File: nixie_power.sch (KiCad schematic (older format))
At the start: 17 parts

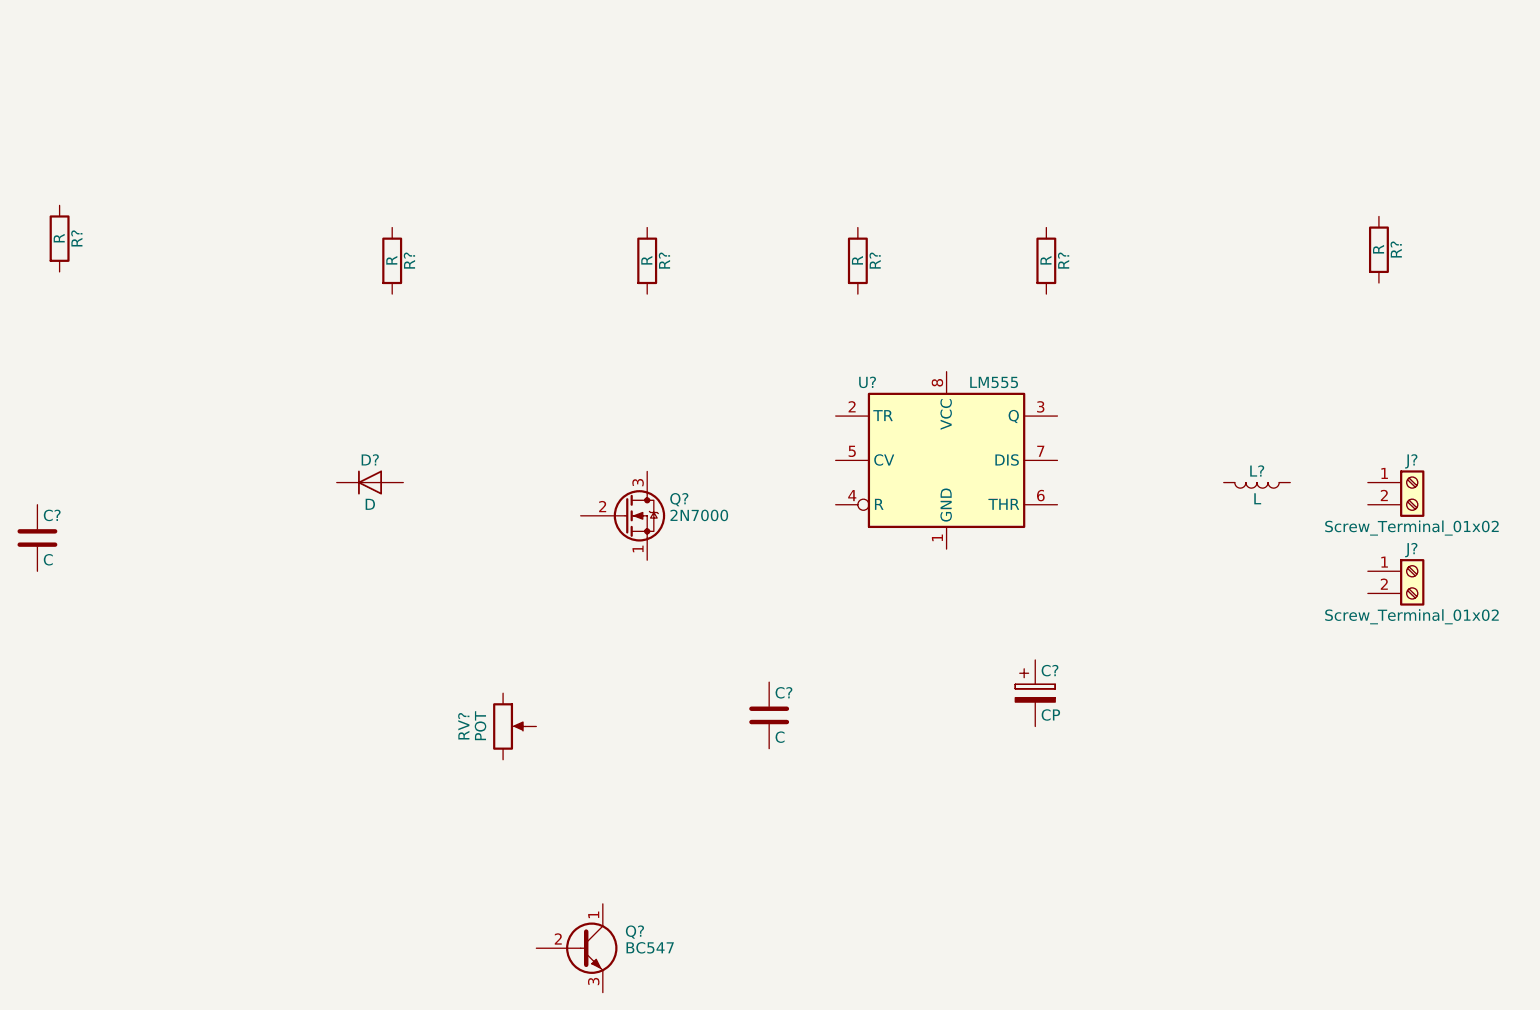
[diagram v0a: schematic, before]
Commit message: 配線をした
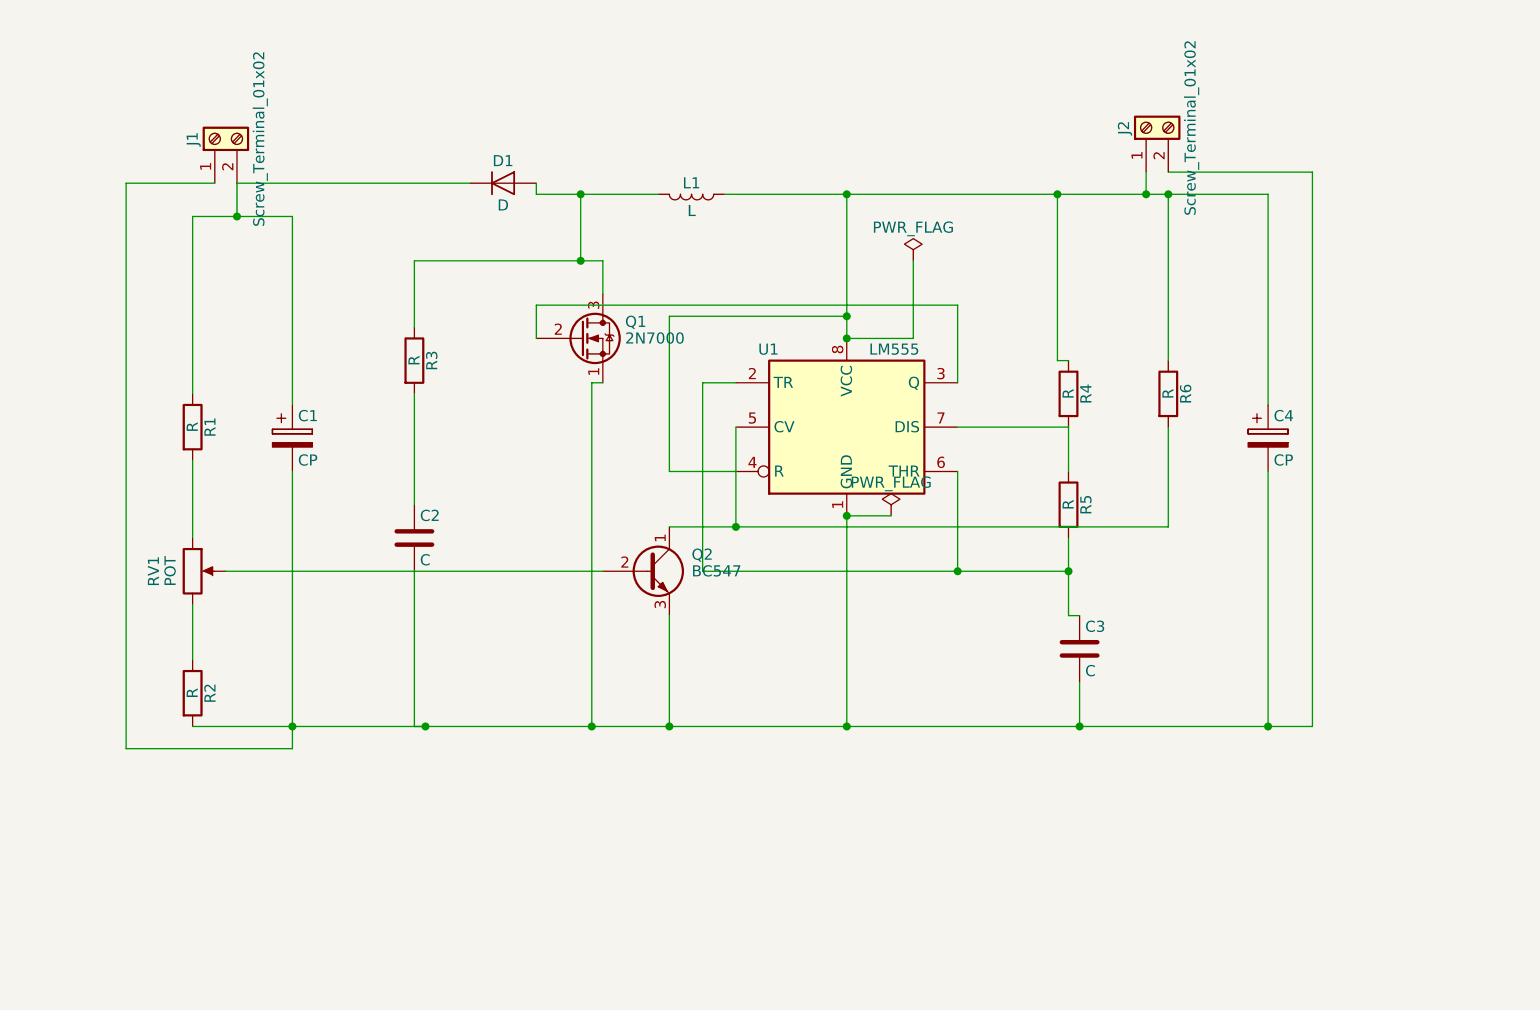
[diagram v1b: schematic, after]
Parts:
- added C4: CP, symbol CP
- gave numbers to parts that had none: 17
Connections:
- net at R1.1: now also C1.1, D1.1 (K), J1.2 (Pin_2)
- net at R1.2: now also RV1.1
- net at R2.1: now also RV1.3
- net at R2.2: now also C1.2, C2.2, C3.2, J1.1 (Pin_1), J2.2 (Pin_2), Q1.1 (S), Q2.3 (E), U1.1 (GND), C4.2
- net at R3.1: now also D1.2 (A), L1.2, Q1.3 (D)
- net at R3.2: now also C2.1
- net at R4.1: now also J2.1 (Pin_1), L1.1, R6.1, U1.4 (R), U1.8 (VCC), C4.1
- net at R4.2: now also R5.1, U1.7 (DIS)
- net at R5.2: now also C3.1, U1.2 (TR), U1.6 (THR)
- net at R6.2: now also Q2.1 (C), U1.5 (CV)
- net at Q2.2 (B): now also RV1.2
- net at Q1.2 (G): now also U1.3 (Q)
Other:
- moved on the sheet: C1, C2, C3, D1, J1, J2, L1, Q1, Q2, R1, R2, R3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
